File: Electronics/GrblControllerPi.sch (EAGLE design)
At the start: 22 parts, among them IC1 ATMEGA168-20P, SW1 SPST_TACT-EVQQ2

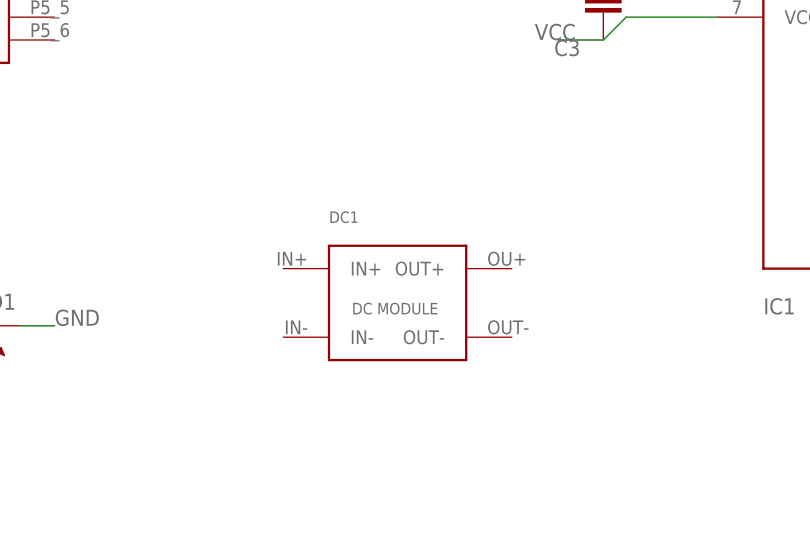
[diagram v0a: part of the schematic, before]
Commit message: Minor Tweaks to hardware + Added GrblpiB+ boards
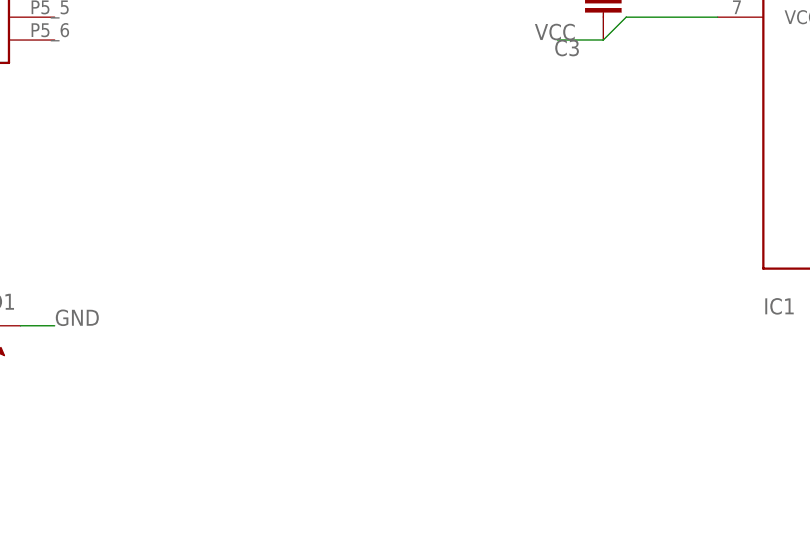
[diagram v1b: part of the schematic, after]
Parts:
- removed DC1: (no value), OpenHardware.co.za:BUCKBOOST
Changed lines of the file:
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@@
 <part name="R4" library="dp_devices" deviceset="RESISTOR" device="-1206" value="1K"/>
 <part name="LED1" library="adafruit" deviceset="LED" device="CHIPLED_1206"/>
-<part name="DC1" library="OpenHardware.co.za" deviceset="BUCKBOOST" device=""/>
 </parts>
 <sheets>
@@
 <instance part="R4" gate="G$1" x="40.64" y="-29.21" rot="R180"/>
 <instance part="LED1" gate="G$1" x="49.53" y="-29.21" rot="R90"/>
-<instance part="DC1" gate="G$1" x="157.48" y="-48.26"/>
 </instances>
 <busses>
